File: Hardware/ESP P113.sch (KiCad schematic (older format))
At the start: 57 parts, among them J1 L_In, J2 R_In, J3 L_Out, J4 R_Out, J5 AC_In, Q1 MJE15032, Q2 MJE15033, Q3 MJE15032, Q4 MJE15033, U1 LM4562

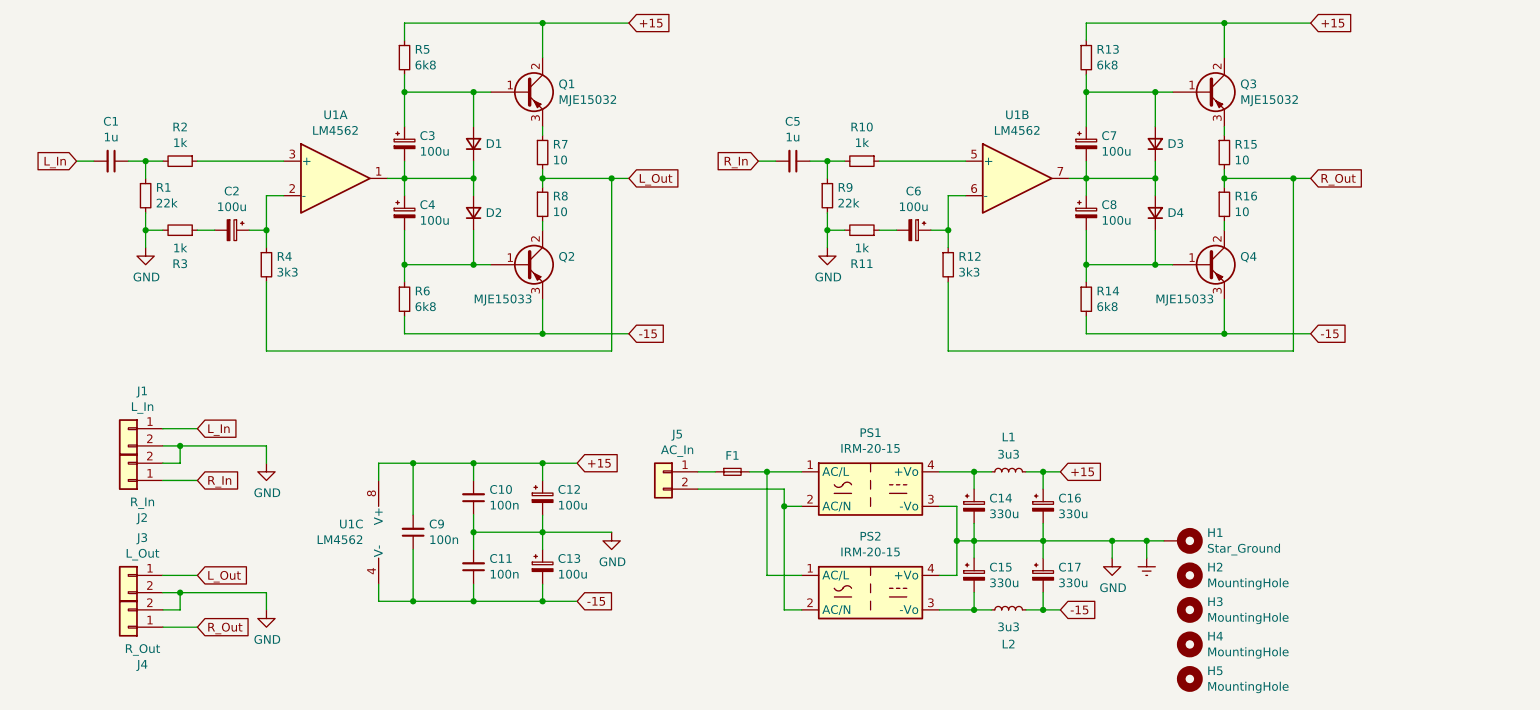
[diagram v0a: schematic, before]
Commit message: Updated to V1.2.
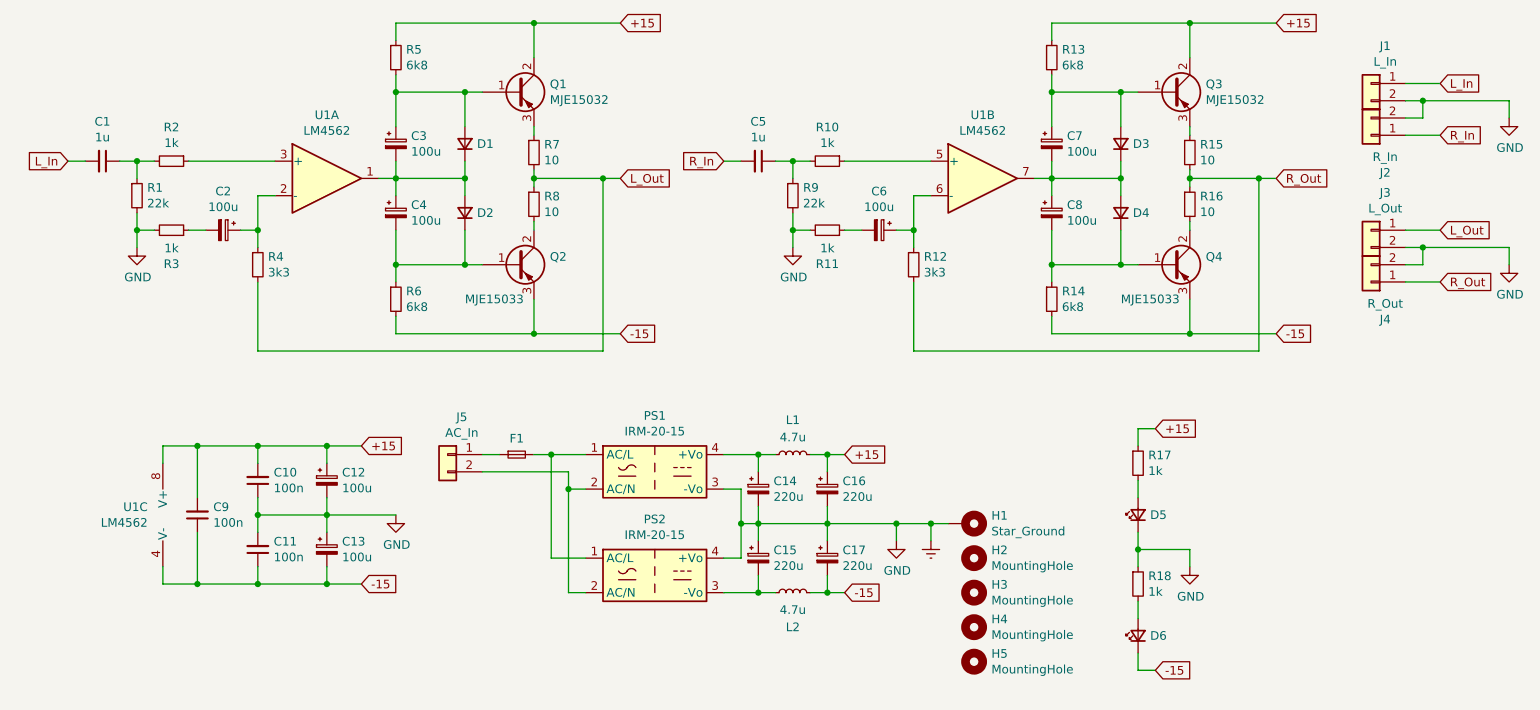
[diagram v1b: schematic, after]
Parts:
- added D5, D6: LED, LED_THT:LED_D3.0mm, symbol Device:LED_Small
- added R17, R18: 1k, Resistor_SMD:R_1206_3216Metric_Pad1.42x1.75mm_HandSolder, symbol Device:R_Small
- C14, C15, C16, C17: value 330u -> 220u
- L1, L2: value 3u3 -> 4.7u; footprint Inductor_THT:L_Radial_D12.5mm_P9.00mm_Fastron_09HCP -> Inductor_SMD:L_Taiyo-Yuden_NR-80xx_HandSoldering
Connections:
- net +15: now also R17.1
- net -15: now also D6.1 (K)
- net Earth: now also D5.1 (K), R18.1
- new net: D5.2 (A), R17.2
- new net: D6.2 (A), R18.2
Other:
- moved on the sheet: C1, C10, C11, C12, C13, C14, C15, C16, C17, C2, C3, C4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
